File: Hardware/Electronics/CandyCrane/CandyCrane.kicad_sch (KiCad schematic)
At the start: 24 parts, among them J1 Screw_Terminal_01x02, J10 Conn_01x03, J11 Conn_01x04, J5 Conn_01x02, J6 Conn_01x02, J7 Conn_01x05, J8 Conn_01x05, J9 Conn_01x05, M1 ESP32_DevKitC-30Pin, U1 ULN2003, U2 BA7806, U3 ULN2003, U4 AP1117-33

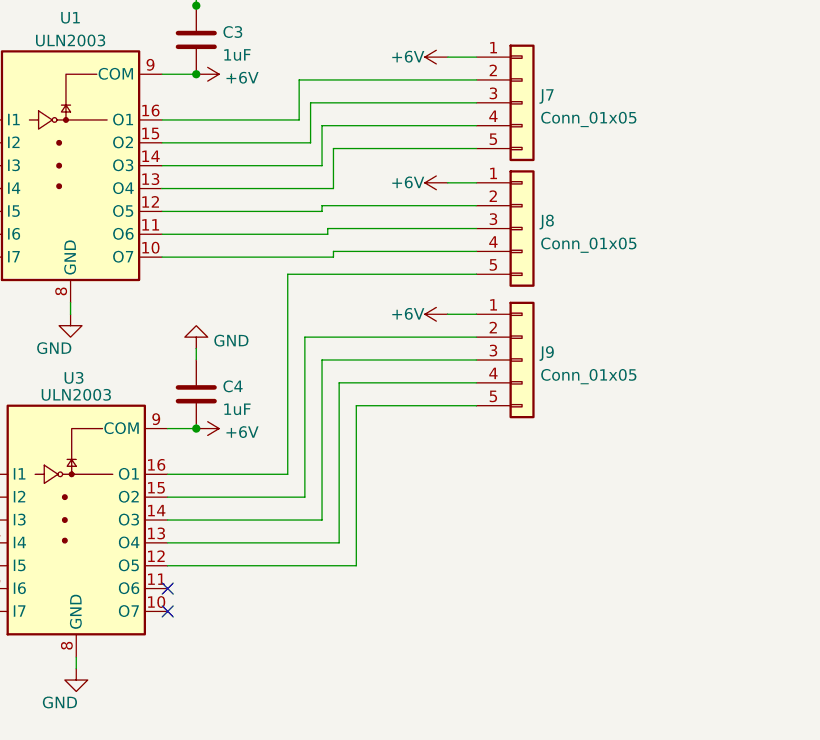
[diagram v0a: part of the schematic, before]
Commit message: updates
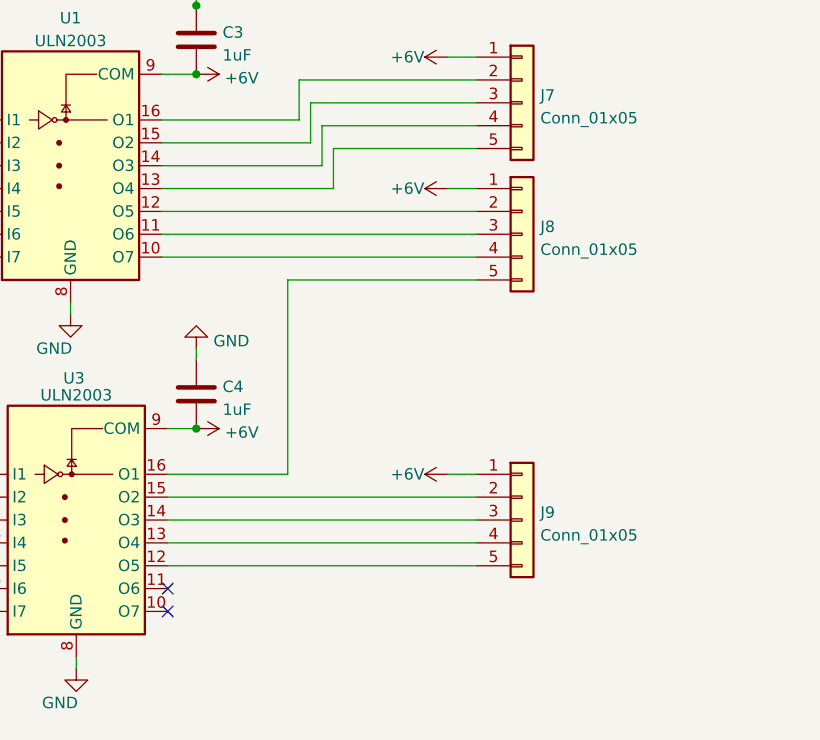
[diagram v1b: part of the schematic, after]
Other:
- moved on the sheet: J8, J9
